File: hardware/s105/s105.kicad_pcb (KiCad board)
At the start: 2 copper layers, 86 x 159 mm, 410 parts, among them J1 Conn_01x06, P1 368255-2, Q1 BC847C, Q10 BC847C, Q11 BC847C, Q12 BC847C, Q13 BC847C, Q14 BC847C, Q15 BC847C, Q16 BC847C, Q17 BC847C, Q18 BC847C, Q2 BC847C, Q20 BC847C, Q21 BC847C, Q22 BC847C, Q23 BC847C, Q3 BC847C, Q4 ., Q5 ., Q6 BC847C, Q7 BC847C, Q8 BC847C, Q9 BC847C, U1 case only, U2 STM32F427VGT6, U4 case only, X1 8MHz 20pF

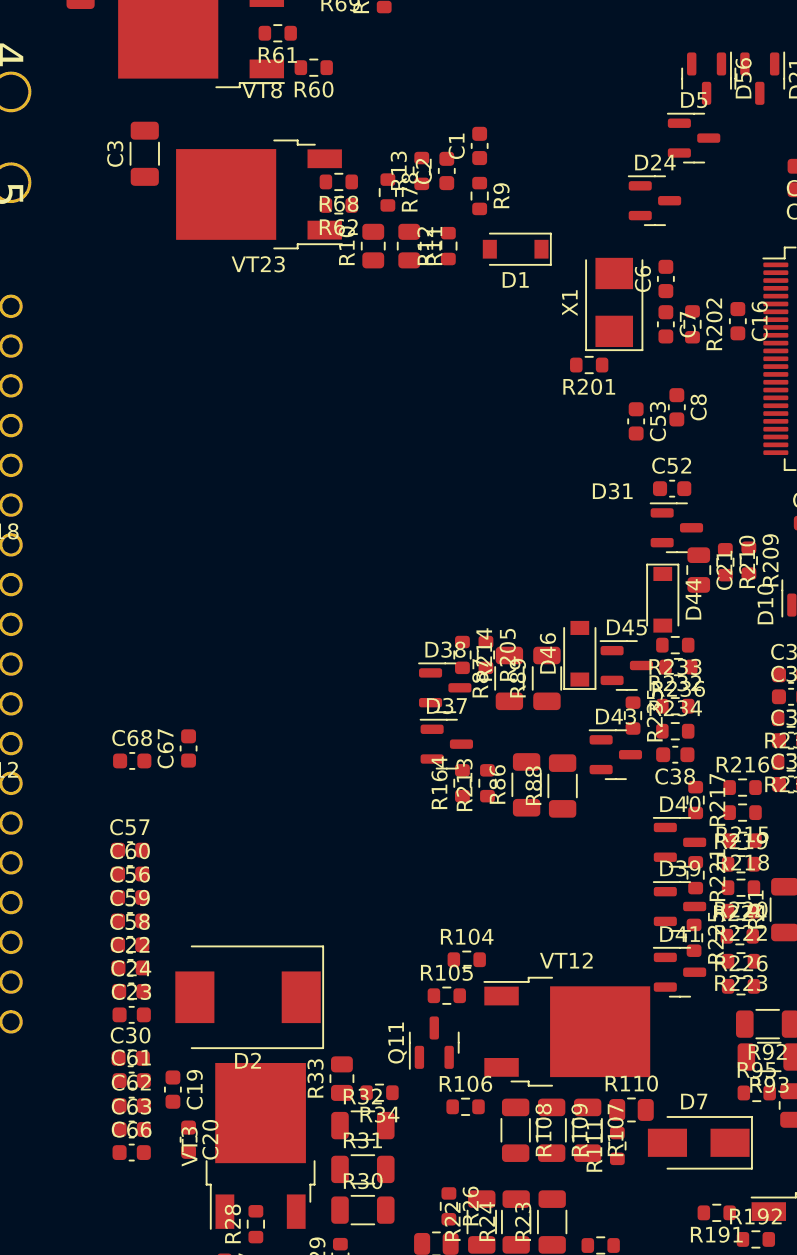
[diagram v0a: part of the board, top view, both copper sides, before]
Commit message: заполняем плату дальше
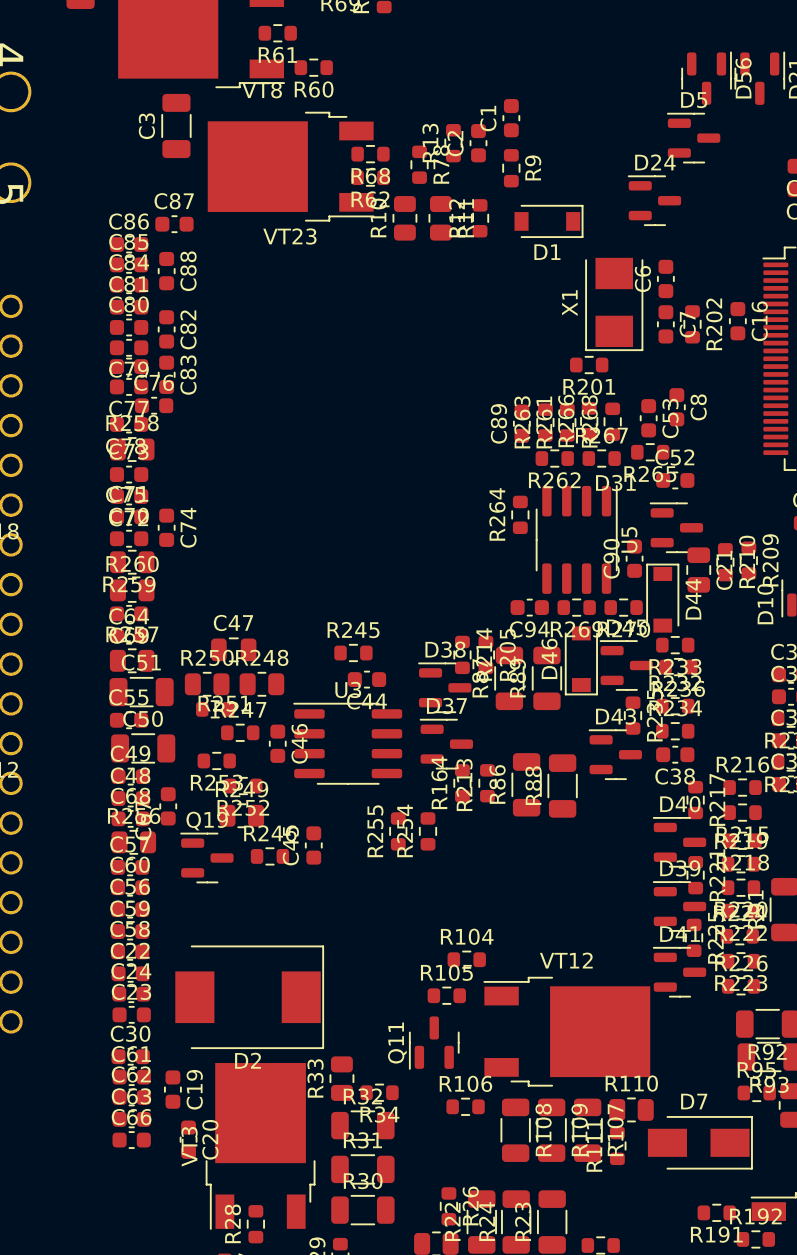
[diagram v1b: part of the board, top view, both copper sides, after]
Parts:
- added C44: C0603, Capacitor_SMD:C_0603_1608Metric, F.Cu at (86.6, 163.0)
- added C45: C0603, Capacitor_SMD:C_0603_1608Metric, F.Cu at (83.2, 173.6)
- added C46: C0603, Capacitor_SMD:C_0603_1608Metric, F.Cu at (80.9, 167.1)
- added C47: C0805, Capacitor_SMD:C_0805_2012Metric, F.Cu at (78.1, 161.1)
- added C48: C0603, Capacitor_SMD:C_0603_1608Metric, F.Cu at (71.5, 170.6)
- added C49: C0603, Capacitor_SMD:C_0603_1608Metric, F.Cu at (71.5, 169.2)
- added C50: C1206, Capacitor_SMD:C_1206_3216Metric, F.Cu at (72.3, 167.4)
- added C51: C1206, Capacitor_SMD:C_1206_3216Metric, F.Cu at (72.2, 163.8)
- added C55: C0603, Capacitor_SMD:C_0603_1608Metric, F.Cu at (71.4, 165.6)
- added C64: C0603, Capacitor_SMD:C_0603_1608Metric, F.Cu at (71.4, 160.2)
- added C69: 100nF, Capacitor_SMD:C_0603_1608Metric, F.Cu at (71.4, 158.8)
- added C70: C0603, Capacitor_SMD:C_0603_1608Metric, F.Cu at (71.4, 154.0)
- added C71: C0603, Capacitor_SMD:C_0603_1608Metric, F.Cu at (71.4, 152.6)
- added C72: 100nF, Capacitor_SMD:C_0603_1608Metric, F.Cu at (71.4, 151.3)
- added C73: C0603, Capacitor_SMD:C_0603_1608Metric, F.Cu at (71.4, 149.9)
- added C74: 100nF, Capacitor_SMD:C_0603_1608Metric, F.Cu at (73.8, 153.3)
- added C75: 100nF, Capacitor_SMD:C_0603_1608Metric, F.Cu at (71.4, 146.7)
- added C76: 100nF, Capacitor_SMD:C_0603_1608Metric, F.Cu at (73.0, 145.5)
- added C77: 100nF, Capacitor_SMD:C_0603_1608Metric, F.Cu at (71.4, 144.3)
- added C78: C0603, Capacitor_SMD:C_0603_1608Metric, F.Cu at (71.4, 143.0)
- added C79: 100nF, Capacitor_SMD:C_0603_1608Metric, F.Cu at (71.4, 141.8)
- added C80: C0603, Capacitor_SMD:C_0603_1608Metric, F.Cu at (71.4, 140.5)
- added C81: C0603, Capacitor_SMD:C_0603_1608Metric, F.Cu at (71.4, 139.2)
- added C82: C0603, Capacitor_SMD:C_0603_1608Metric, F.Cu at (73.8, 140.6)
- added C83: C0603, Capacitor_SMD:C_0603_1608Metric, F.Cu at (73.8, 143.5)
- added C84: C0603, Capacitor_SMD:C_0603_1608Metric, F.Cu at (71.4, 137.8)
- added C85: C0603, Capacitor_SMD:C_0603_1608Metric, F.Cu at (71.4, 136.5)
- added C86: C0603, Capacitor_SMD:C_0603_1608Metric, F.Cu at (71.4, 135.2)
- added C87: C0603, Capacitor_SMD:C_0603_1608Metric, F.Cu at (74.3, 133.9)
- added C88: C0603, Capacitor_SMD:C_0603_1608Metric, F.Cu at (73.8, 136.9)
- added C89: C0603, Capacitor_SMD:C_0603_1608Metric, F.Cu at (96.5, 146.7)
- added C90: C0603, Capacitor_SMD:C_0603_1608Metric, F.Cu at (103.7, 155.3)
- added C94: C0603, Capacitor_SMD:C_0603_1608Metric, F.Cu at (97.0, 158.4)
- added Q19: ., Package_TO_SOT_SMD:SOT-23, F.Cu at (76.4, 174.4)
- added R245: 4.7k, Resistor_SMD:R_0603_1608Metric, F.Cu at (85.7, 161.3)
- added R246: 82k, Resistor_SMD:R_0603_1608Metric, F.Cu at (80.4, 174.3)
- added R247: 4.7k, Resistor_SMD:R_0603_1608Metric, F.Cu at (78.5, 166.4)
- added R248: 10k, Resistor_SMD:R_0805_2012Metric, F.Cu at (79.9, 163.3)
- added R249: 10k, Resistor_SMD:R_0805_2012Metric, F.Cu at (78.6, 171.7)
- added R250: 10k, Resistor_SMD:R_0805_2012Metric, F.Cu at (76.4, 163.3)
- added R251: 4.7k, Resistor_SMD:R_0603_1608Metric, F.Cu at (76.9, 164.9)
- added R252: 4.7k, Resistor_SMD:R_0603_1608Metric, F.Cu at (78.7, 169.8)
- added R253: 4.7k, Resistor_SMD:R_0603_1608Metric, F.Cu at (77.0, 168.2)
- added R254: 4.7k, Resistor_SMD:R_0603_1608Metric, F.Cu at (90.5, 172.7)
- added R255: NM, Resistor_SMD:R_0603_1608Metric, F.Cu at (88.6, 172.7)
- added R256: 0, Resistor_SMD:R_0805_2012Metric, F.Cu at (71.7, 173.4)
- added R257: 0, Resistor_SMD:R_0805_2012Metric, F.Cu at (71.6, 161.8)
- added R258: 0, Resistor_SMD:R_0805_2012Metric, F.Cu at (71.6, 148.3)
- added R259: 0, Resistor_SMD:R_0805_2012Metric, F.Cu at (71.6, 155.5)
- added R260: 0, Resistor_SMD:R_0805_2012Metric, F.Cu at (71.6, 157.3)
- added R261: NM, Resistor_SMD:R_0603_1608Metric, F.Cu at (99.4, 146.6)
- added R262: MN, Resistor_SMD:R_0603_1608Metric, F.Cu at (98.6, 148.9)
- added R263: 3k, Resistor_SMD:R_0603_1608Metric, F.Cu at (98.0, 146.6)
- added R264: 3k, Resistor_SMD:R_0603_1608Metric, F.Cu at (96.4, 152.5)
- added R265: MN, Resistor_SMD:R_0603_1608Metric, F.Cu at (104.7, 148.5)
- added R266: MN, Resistor_SMD:R_0603_1608Metric, F.Cu at (100.8, 146.5)
- added R267: MN, Resistor_SMD:R_0603_1608Metric, F.Cu at (101.6, 148.9)
- added R268: MN, Resistor_SMD:R_0603_1608Metric, F.Cu at (102.3, 146.5)
- added R269: 10k, Resistor_SMD:R_0603_1608Metric, F.Cu at (100.0, 158.4)
- added R270: MN, Resistor_SMD:R_0603_1608Metric, F.Cu at (103.0, 158.4)
- added U3: case only, Package_SO:SOIC-8_3.9x4.9mm_P1.27mm, F.Cu at (85.4, 167.1)
- added U5: case only, Package_SO:SOIC-8_3.9x4.9mm_P1.27mm, F.Cu at (100.0, 154.1)
- moved C67 3.92 mm to (73.9, 171.1)
- moved C68 3.70 mm to (71.5, 171.9)
- moved C1 2.69 mm to (95.8, 127.1)
- moved D1 2.69 mm to (98.1, 133.7)
- moved R10 2.69 mm to (89.0, 133.5)
- moved R11 2.69 mm to (91.3, 133.5)
- moved R12 2.69 mm to (93.8, 133.5)
- moved R13 2.69 mm to (92.1, 128.7)
- moved R78 2.69 mm to (90.0, 130.1)
- moved R9 2.69 mm to (95.8, 130.3)
- moved C2 2.69 mm to (93.7, 128.7)
- moved C3 2.69 mm to (74.4, 127.6)
- moved VT23 2.69 mm to (81.7, 130.2)
- moved R62 2.69 mm to (86.8, 130.9)
- moved R68 2.69 mm to (86.8, 129.4)
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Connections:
- J1 pad 5: /MCU/5V -> +5V
- P1 pad 12: unconnected-(P1-Pad12) -> Net-(C48-Pad1)
- P1 pad 14: unconnected-(P1-Pad14) -> Net-(C55-Pad1)
- P1 pad 17: GND -> /GNDA
- P1 pad 20: GND -> /GNDA
- P1 pad 35: GND -> /GNDA
- P1 pad 36: GND -> /GNDA
- P1 pad 51: GND -> /GNDA
- P1 pad 52: GND -> /GNDA
- P1 pad 53: GND -> /GNDA
- P1 pad 54: GND -> /GNDA
- U2 pad 29: /MCU/PA4 -> /PA4
- U2 pad 47: /MCU/PB10 -> /PB10
- U2 pad 5: /MCU/PE6 -> /PE6
